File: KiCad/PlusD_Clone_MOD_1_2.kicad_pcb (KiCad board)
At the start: 2 copper layers, 98.6 x 99.1 mm, 65 parts, among them IC10 74LS27, IC12 L7805, IC5 74LS06, IC6 74LS126, IC9 74LS00, J1 ZX_CONNECTOR_GENERIC_SORTED, J2 FDD_CONNECTOR, J3 PARALLEL_CONNECTOR, J4 KEMPSTON, SW1 RESET, SW2 NMI, SW3 ROMSEL_JOY, SW4 ZX_SEL, SW5 ABBA, U1 WD1772, U11 GAL22V10, U2 27E257, U3 6264, U4 PAL20L8, U7 74LS374, U8 74LS175, Y1 8.000Mhz

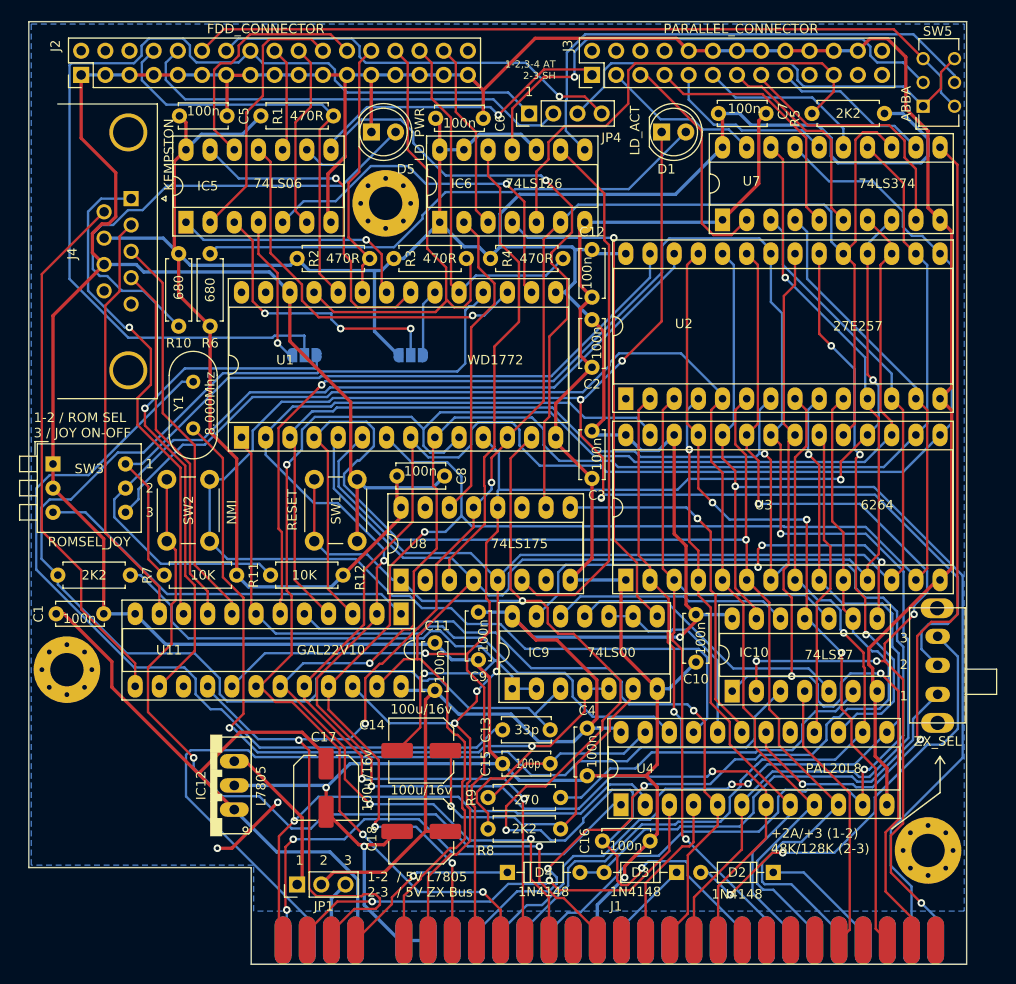
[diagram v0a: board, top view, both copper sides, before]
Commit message: Add files via upload
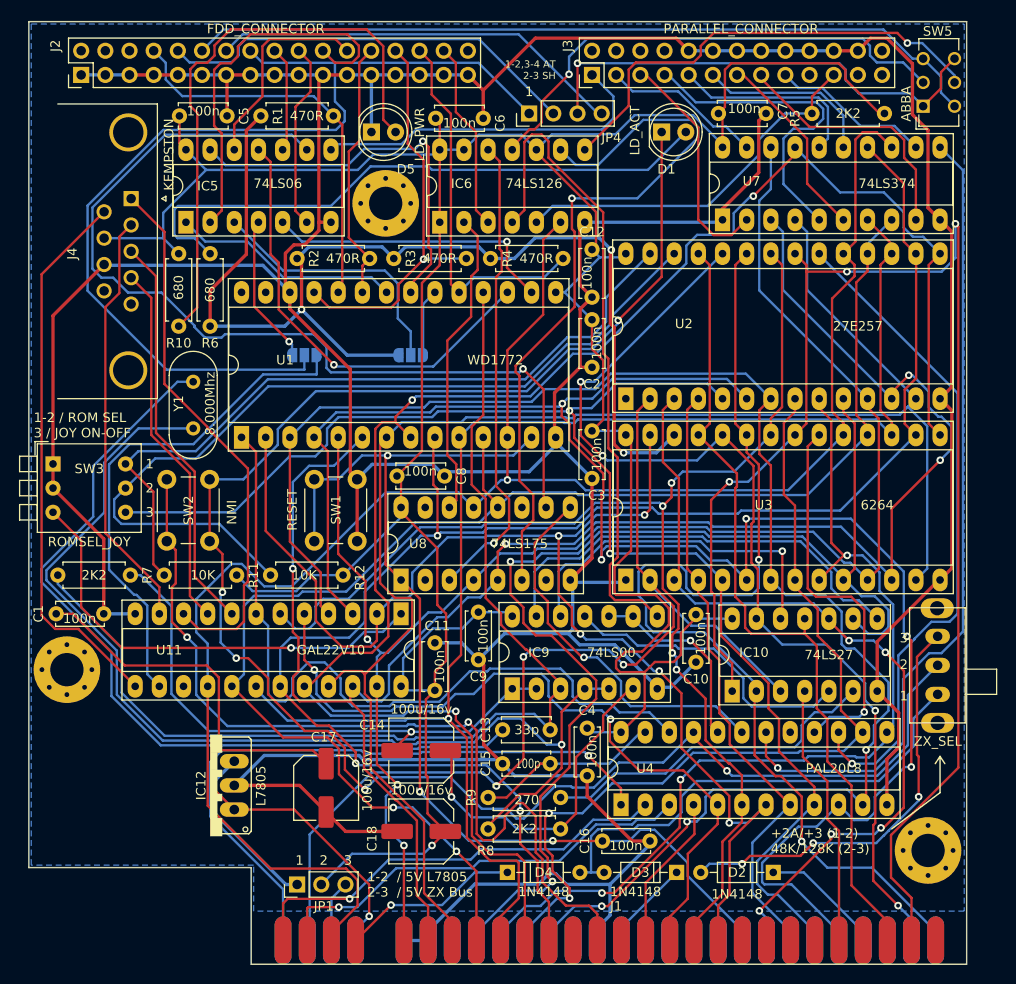
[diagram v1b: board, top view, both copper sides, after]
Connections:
- net /SELROM3 renamed Net-(D3-Pad2)
- net /SELROM48 renamed Net-(D2-Pad2)
- net 9V renamed +9V
- C10 pad 2: 5V -> +5V
- C11 pad 2: 5V -> +5V
- C12 pad 2: 5V -> +5V
- C18 pad 1: 5V -> +5V
- C2 pad 2: 5V -> +5V
- C3 pad 2: 5V -> +5V
- C4 pad 2: 5V -> +5V
- C5 pad 2: 5V -> +5V
- C6 pad 2: 5V -> +5V
- C7 pad 2: 5V -> +5V
- C8 pad 2: 5V -> +5V
- C9 pad 2: 5V -> +5V
- IC10 pad 14: 5V -> +5V
- IC5 pad 14: 5V -> +5V
- IC6 pad 1: 5V -> +5V
- IC6 pad 10: 5V -> +5V
- IC6 pad 13: 5V -> +5V
- IC6 pad 14: 5V -> +5V
- IC9 pad 14: 5V -> +5V
- J4 pad 7: 5V -> +5V
- JP1 pad 2: 5V -> +5V
- R10 pad 2: 5V -> +5V
- R11 pad 2: 5V -> +5V
- R12 pad 2: 5V -> +5V
- R5 pad 2: 5V -> +5V
- U1 pad 15: 5V -> +5V
- U11 pad 24: 5V -> +5V
- U2 pad 28: 5V -> +5V
- U3 pad 28: 5V -> +5V
- U4 pad 24: 5V -> +5V
- U7 pad 20: 5V -> +5V
- U8 pad 16: 5V -> +5V
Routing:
- net +5V: track 0.00 -> 356.3 mm, vias 0 -> 1
- net 5V: track 402.8 -> 116.9 mm, vias 1 -> 3
- net A10: track 97.8 -> 151.8 mm, vias 2 -> 3
- net RD: track 182.8 -> 134.6 mm, vias 2 -> 4
- net A4: track 150.8 -> 187.0 mm, vias 1 -> 5
- net A0: track 93.7 -> 123.4 mm
- net Net-(IC5-Pad9): track 70.5 -> 99.9 mm
- net D1: track 170.0 -> 193.5 mm, vias 3 -> 4
- net RESET: track 133.6 -> 110.8 mm
- net Net-(IC9-Pad4): track 91.8 -> 114.4 mm, vias 2 -> 1
- net Net-(D1-Pad1): track 213.3 -> 190.9 mm, vias 3 -> 5
- net Net-(IC6-Pad9): track 56.6 -> 78.4 mm, vias 0 -> 1
- net A12: track 133.1 -> 112.2 mm, vias 1 -> 3
- net GND: track 591.0 -> 570.9 mm, vias 5 -> 0
- net Net-(C13-Pad2): track 134.7 -> 114.8 mm
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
